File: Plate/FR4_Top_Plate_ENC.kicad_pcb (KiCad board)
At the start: 2 copper layers, 139.1 x 107.7 mm, 35 parts, among them SW1 SW_PUSH, SW10 SW_PUSH, SW11 SW_PUSH, SW12 SW_PUSH, SW13 SW_PUSH, SW14 SW_PUSH, SW15 SW_PUSH, SW16 SW_PUSH, SW17 SW_PUSH, SW18 SW_PUSH, SW19 SW_PUSH, SW2 SW_PUSH, SW20 SW_PUSH, SW21 SW_PUSH, SW22 SW_PUSH, SW23 SW_PUSH, SW24 SW_PUSH, SW25 SW_PUSH, SW26 SW_PUSH, SW27 SW_PUSH, SW28 SW_PUSH, SW29 SW_PUSH, SW3 SW_PUSH, SW30 Rotary_Encoder_Switch, SW4 SW_PUSH, SW5 SW_PUSH, SW6 SW_PUSH, SW7 SW_PUSH, SW8 SW_PUSH, SW9 SW_PUSH

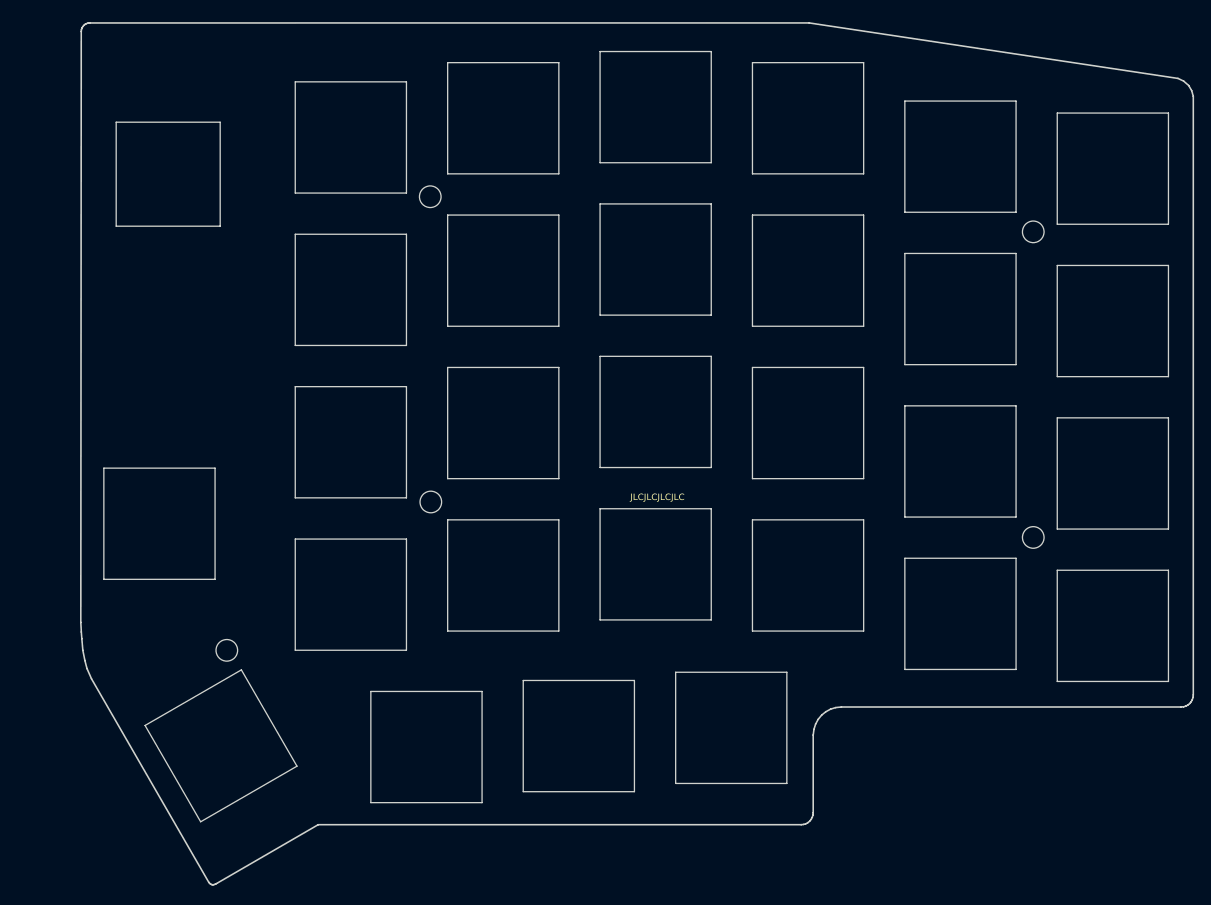
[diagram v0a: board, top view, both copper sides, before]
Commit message: Revert "Merge pull request #53 from TweetyDaBird/release"
This reverts commit d5395b9879702c31b6de7b44cd45c4487da02165, reversing
changes made to 721366541e1b3daa08e8a27e832954bcb38f5212.

# Conflicts:
#	.gitignore
#	Lotus 58 Classic/v1.26/Lotus58_Glow_126.kicad_pcb
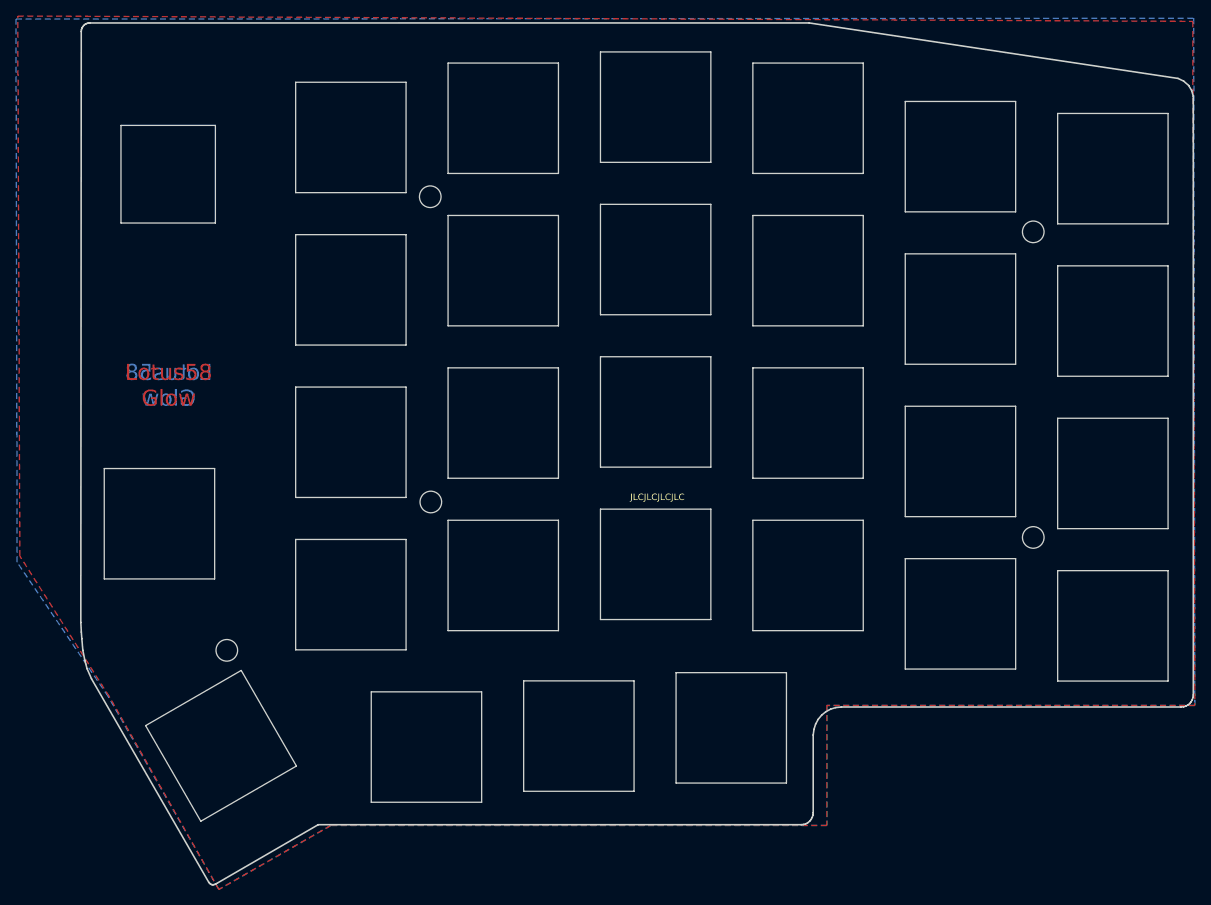
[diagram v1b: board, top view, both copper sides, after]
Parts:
- SW1, SW10, SW11, SW12, SW13, SW14, SW15, SW16, SW17, SW18, SW19, SW2, SW20, SW21, SW22, SW23, SW24, SW25, SW26, SW27, SW28, SW29, SW3, SW4, SW5, SW6, SW7, SW8, SW9: footprint Keyboard_Plate:SW_MX_Plate_Placeholder_nodrill_NOBORDER_13,9 -> Keyboard Library:Cherry_MX_Plate_Hole_Placeholder
- SW30: footprint Keyboard Encoders:Encoder_Plate_Placeholder_nodrill -> Keyboard Library:RotaryEncoder_PlateHole_Placeholder
- turned SW30 to -90 degrees
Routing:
- added copper zone on B.Cu, net (none)
- added copper zone on F.Cu, net (none)
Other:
- board text added: "Lotus58 Glow"

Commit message: Updated plates
Plates now have no copper layer, both preparing for wireless, and to avoid scratches/shorting, if OLED etc. is not soldered with flat pads.
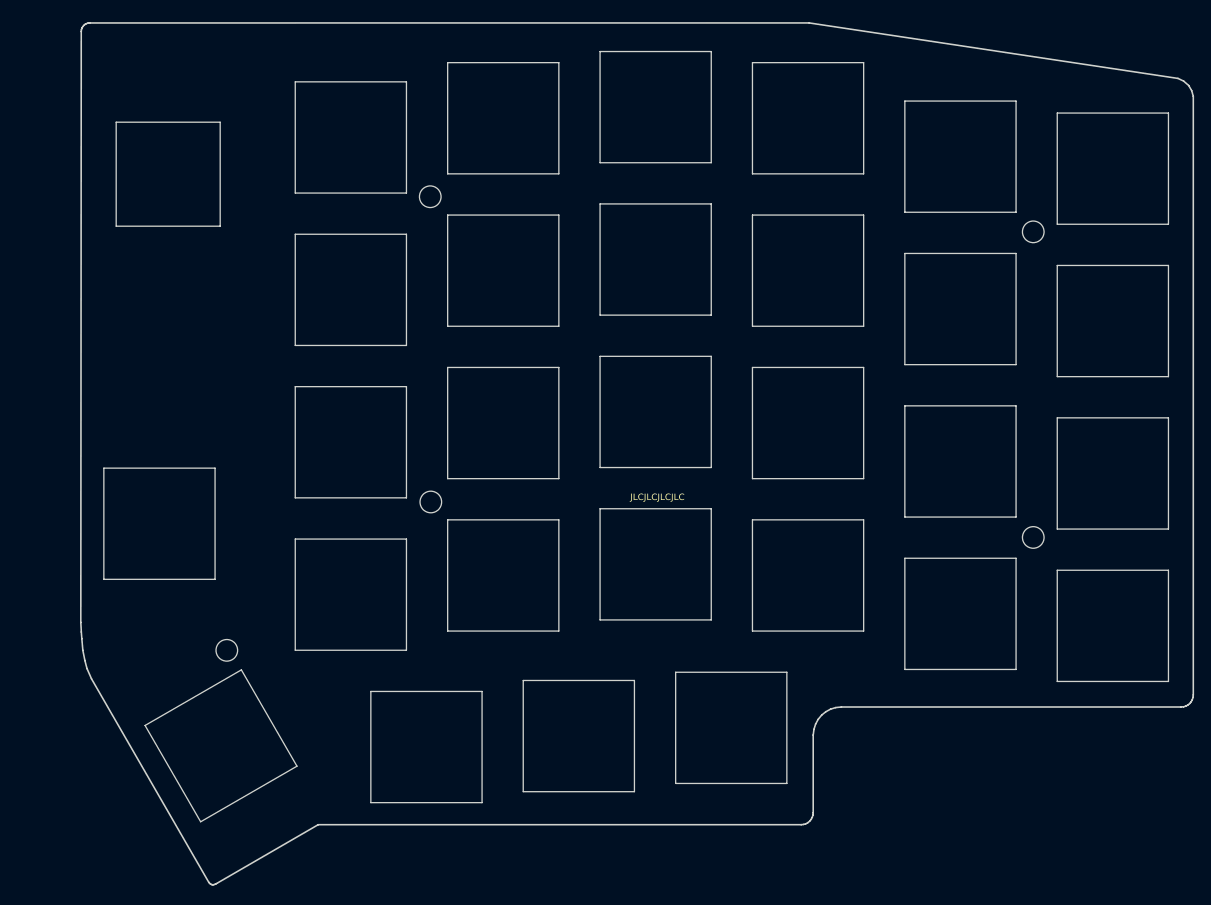
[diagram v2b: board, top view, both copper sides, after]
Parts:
- SW1, SW10, SW11, SW12, SW13, SW14, SW15, SW16, SW17, SW18, SW19, SW2, SW20, SW21, SW22, SW23, SW24, SW25, SW26, SW27, SW28, SW29, SW3, SW4, SW5, SW6, SW7, SW8, SW9: footprint Keyboard Library:Cherry_MX_Plate_Hole_Placeholder -> Keyboard_Plate:SW_MX_Plate_Placeholder_nodrill_NOBORDER_13,9
- SW30: footprint Keyboard Library:RotaryEncoder_PlateHole_Placeholder -> Keyboard Encoders:Encoder_Plate_Placeholder_nodrill
- turned SW30 to 0 degrees
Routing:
- removed copper zone on B.Cu, net (none)
- removed copper zone on F.Cu, net (none)
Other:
- board text removed: "Lotus58 Glow"
